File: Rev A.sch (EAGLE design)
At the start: 12 parts, among them IC1 LM324N, Q2 TIP41C

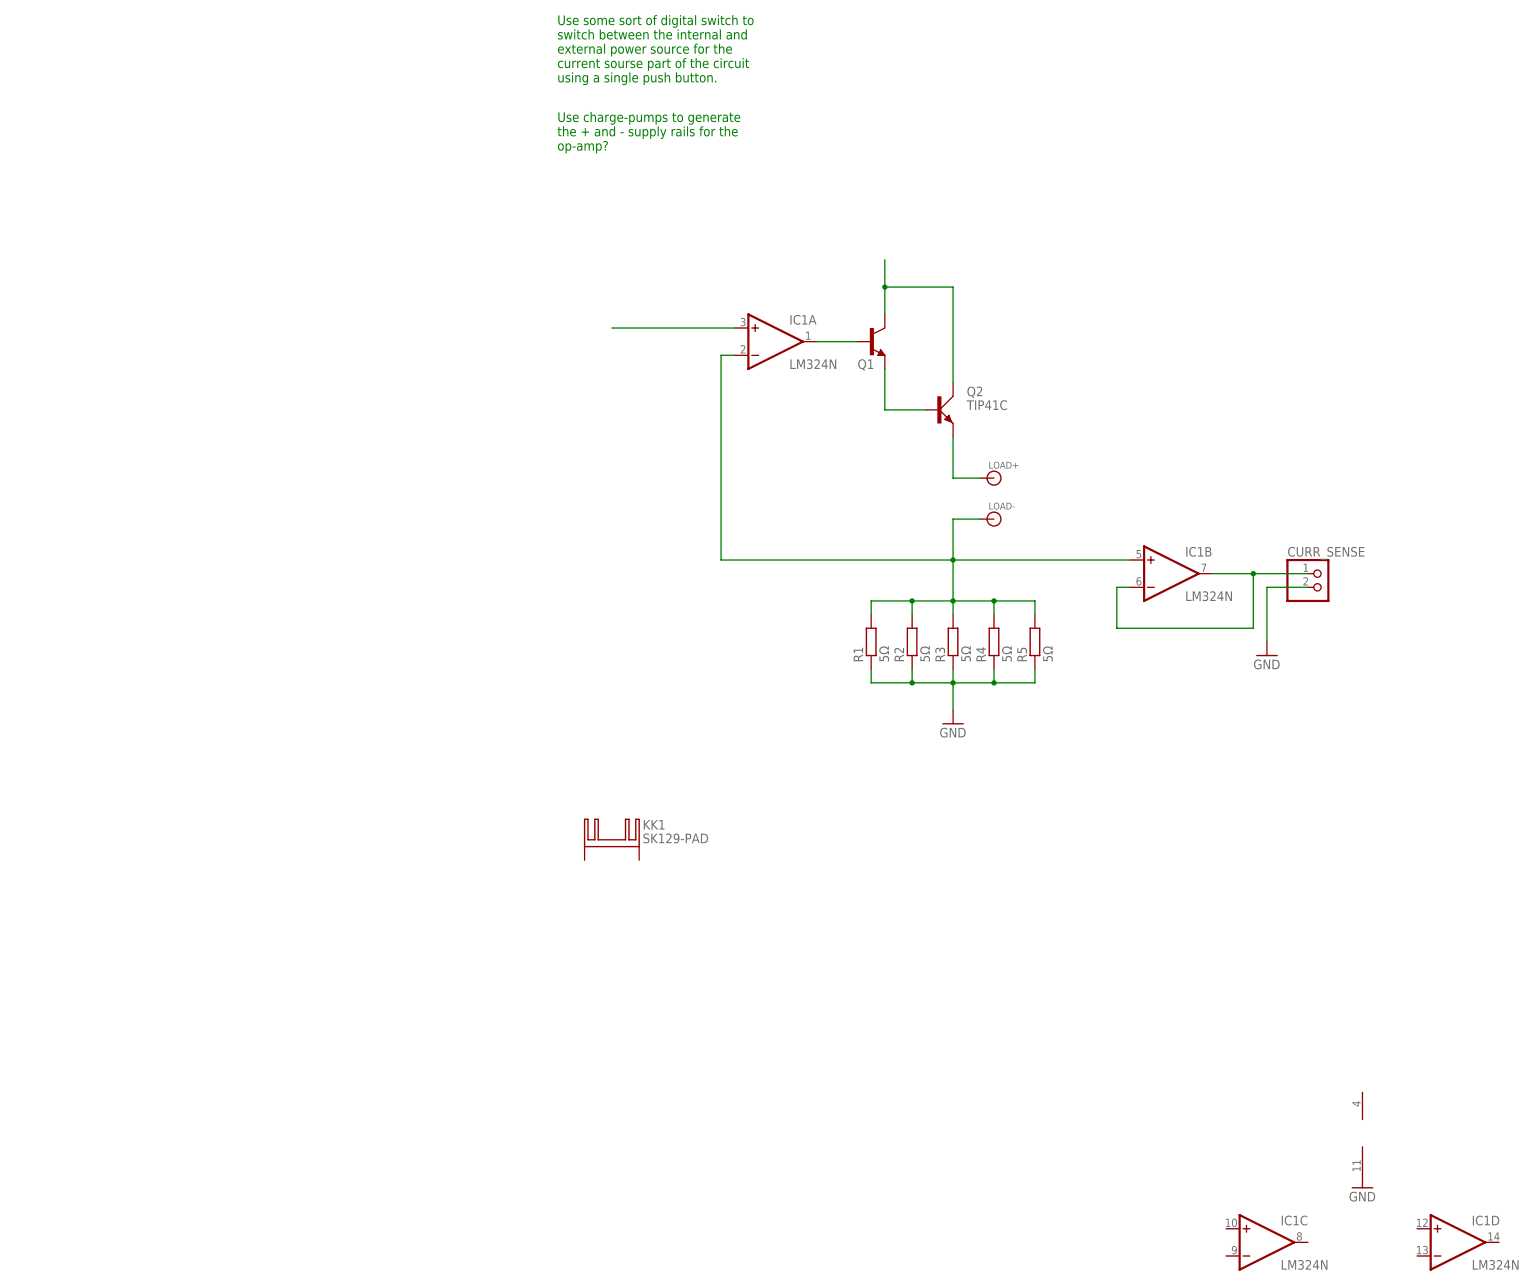
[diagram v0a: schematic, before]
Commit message: Finished the schematic
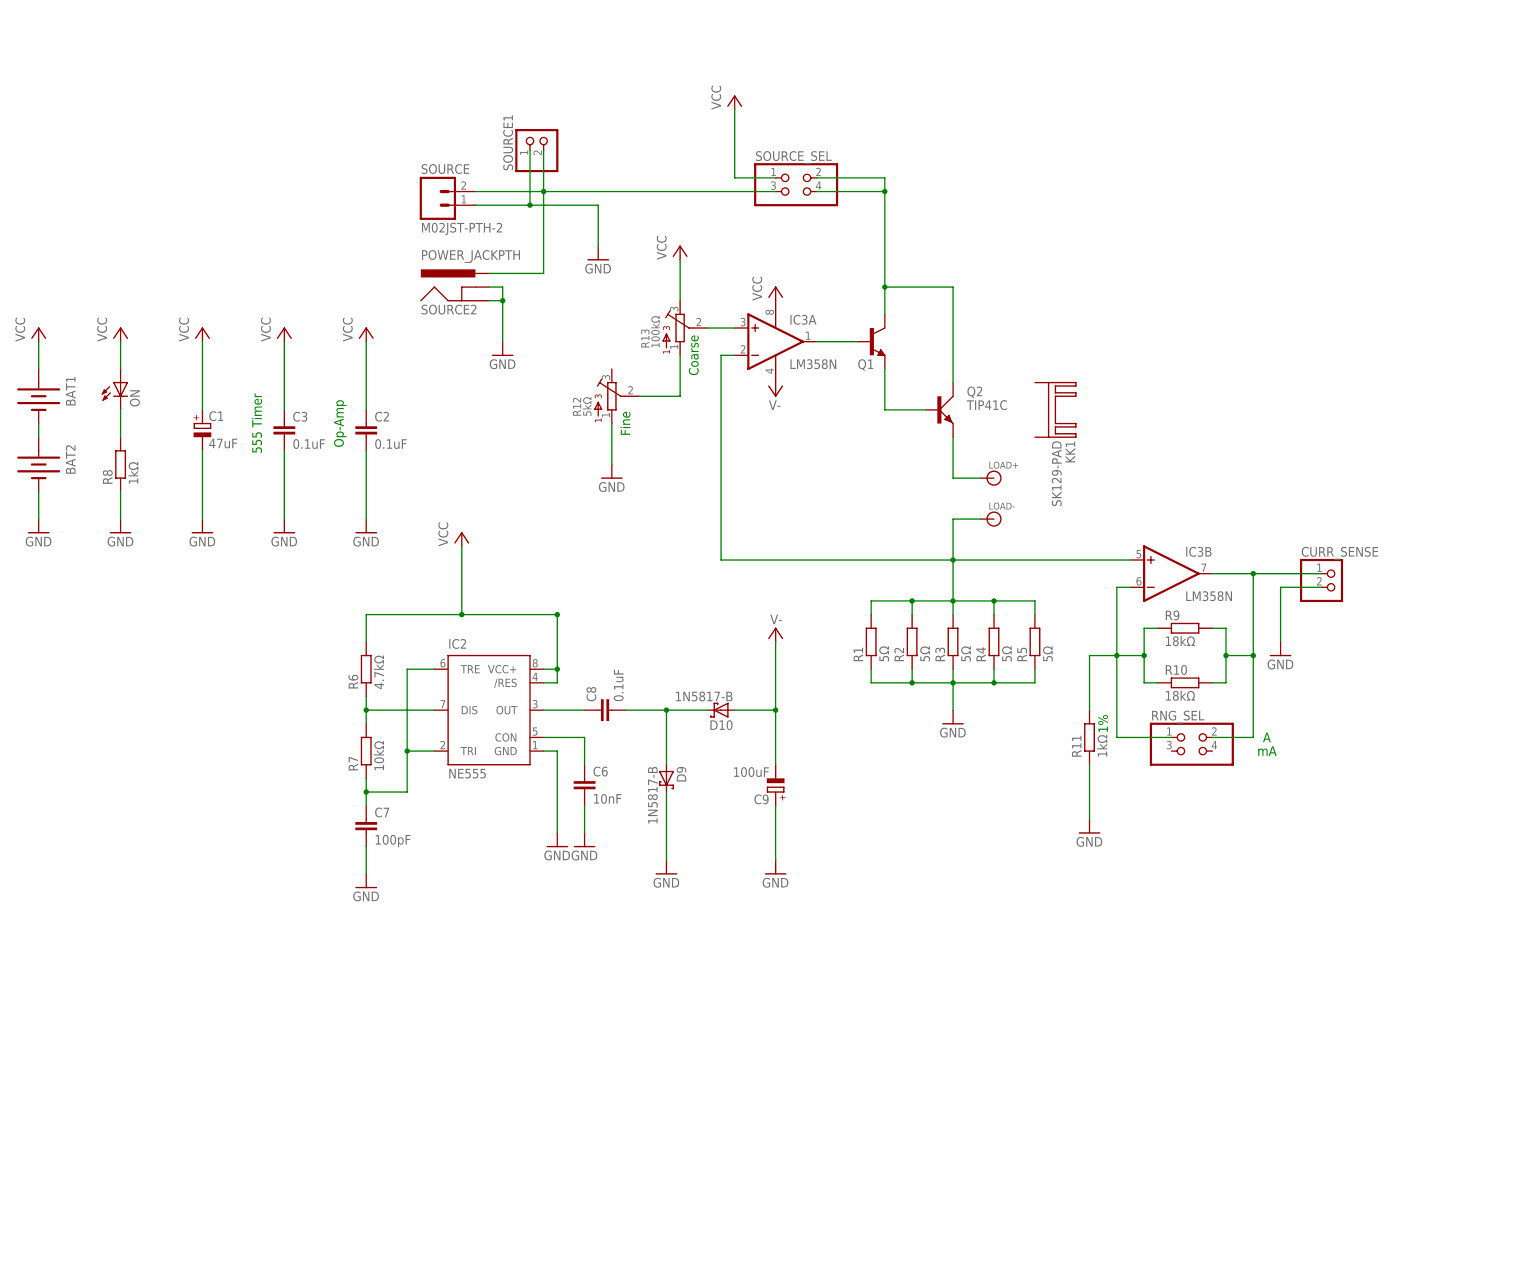
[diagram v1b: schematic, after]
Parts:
- removed IC1: LM324N, linear:LM324N
- added BAT1, BAT2: (no value), SparkFun-Electromechanical:BATTERYAA
- added C1: 47uF, rcl:CPOL-EUE2.5-6
- added C2, C3, C8: 0.1uF, rcl:C-EU050-025X075
- added C6: 10nF, rcl:C-EU050-025X075
- added C7: 100pF, rcl:C-EU025-025X050
- added C9: 100uF, rcl:CPOL-EUE2.5-6
- added D10, D9: 1N5817-B, diode:1N5817-B
- added IC2: NE555, st-microelectronics:NE555
- added IC3: LM358N, linear:LM358N
- added ON: (no value), led:LEDSQR2X5
- added R10, R9: 18kΩ, resistor:R-EU_0207/10
- added R11, R8: 1kΩ, resistor:R-EU_0207/10
- added R12: 5kΩ, bourns:3362U
- added R13: 100kΩ, bourns:3362U
- added R6: 4.7kΩ, resistor:R-EU_0207/10
- added R7: 10kΩ, resistor:R-EU_0207/10
- added RNG_SEL, SOURCE_SEL: (no value), pinhead:PINHD-2X2
- added SOURCE: M02JST-PTH-2, SparkFun-Connectors:M02JST-PTH-2
- added SOURCE1: (no value), pinhead:PINHD-1X2
- added SOURCE2: POWER_JACKPTH, SparkFun-Connectors:POWER_JACKPTH
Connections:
- new net N$10: BAT1.-, BAT2.+
- new net N$13: SOURCE.2, SOURCE1.2, SOURCE2.PWR, SOURCE_SEL.3
- new net N$17: C8.1, IC2.OUT
- new net N$18: C6.1, IC2.CON
- new net N$19: C7.1, IC2.TRE, IC2.TRI, R7.1
- new net N$20: IC2.DIS, R6.1, R7.2
- new net N$25: C8.2, D10.C, D9.A
- new net N$6: ON.C, R8.2
- new net N$8: IC3B.-IN, R10.1, R11.2, R9.1, RNG_SEL.1
- new net N$9: CURR_SENSE.1, IC3B.OUT, R10.2, R9.2, RNG_SEL.2
- new net V-: C9.-, D10.A, IC3P.V-
- new net VCC: BAT1.+, C1.+, C2.1, C3.1, IC2./RES, IC2.VCC+, IC3P.V+, ON.A, R13.3, R6.2, SOURCE_SEL.1
- net CURR_SENSE: now also IC3A.-IN, IC3B.+IN; no longer IC1A.-IN, IC1B.+IN
- net GND: now also BAT2.-, C1.-, C2.2, C3.2, C6.2, C7.2, C9.+, D9.C, IC2.GND, R11.1, R12.1, R8.1, SOURCE.1, SOURCE1.1, SOURCE2.GND, SOURCE2.GNDBREAK; no longer IC1P.V-
- net N$1: now also IC3A.OUT; no longer IC1A.OUT
- net N$3: now also SOURCE_SEL.2, SOURCE_SEL.4
- net N$5: now also R12.2, R13.1; no longer IC1B.-IN, IC1B.OUT
- net N$7: now also IC3A.+IN, R13.2; no longer IC1A.+IN
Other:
- note added: "1%"
- note added: "555 Timer"
- note added: "A"
- note added: "Coarse"
- note added: "Fine"
- note added: "Op-Amp"
- note added: "mA"
- note removed: "Use charge-pumps to generate the + and - supply rails for the op-amp?"
- note removed: "Use some sort of digital switch to switch between the internal and external power source for the current sourse part of the circuit using a single push button."
- moved on the sheet: CURR_SENSE, KK1
